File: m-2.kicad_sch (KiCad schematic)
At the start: 18 parts, among them J503 Bus_M.2_1-2199230-6, M503 Mech_M2_2280_H2.5mm

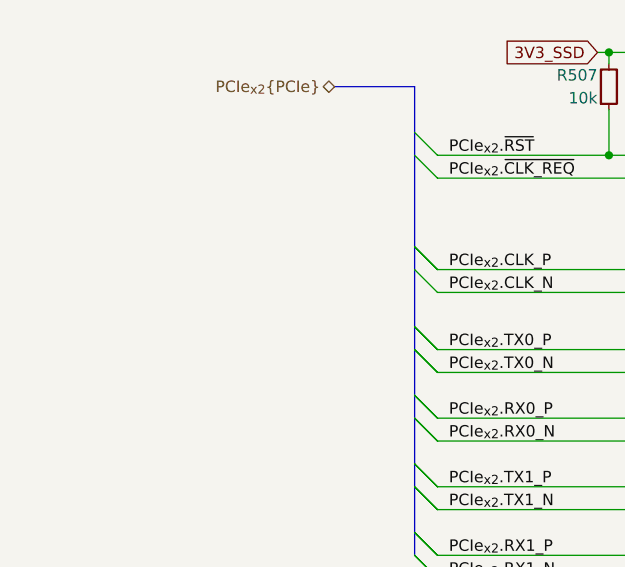
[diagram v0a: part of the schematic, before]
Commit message: [#100765] Update schematic
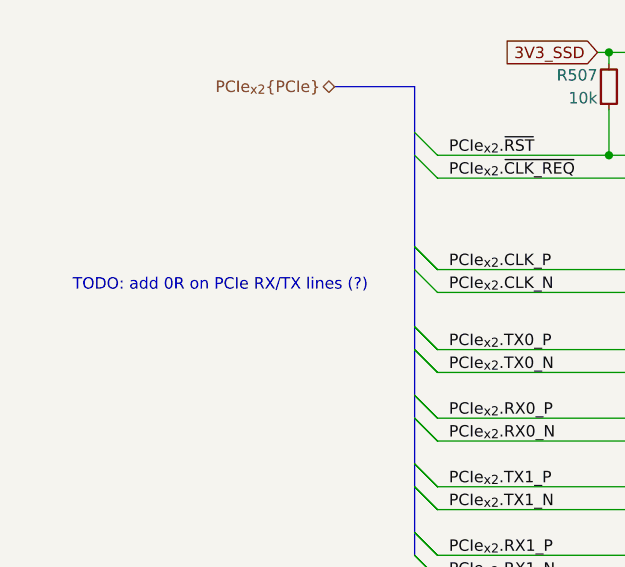
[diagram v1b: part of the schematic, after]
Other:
- note added: "TODO: add 0R on PCIe RX/TX lines (?)"
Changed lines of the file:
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@@
+		)
+	)
+	(text "TODO: add 0R on PCIe RX/TX lines (?)"
+		(exclude_from_sim no)
+		(at 68.58 76.708 0)
+		(effects
+			(font
+				(size 1.27 1.27)
+			)
 		)
 	)
